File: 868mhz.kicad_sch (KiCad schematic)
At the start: 4 parts, among them J2 Conn_Coaxial, U2 RFM95W-868S2

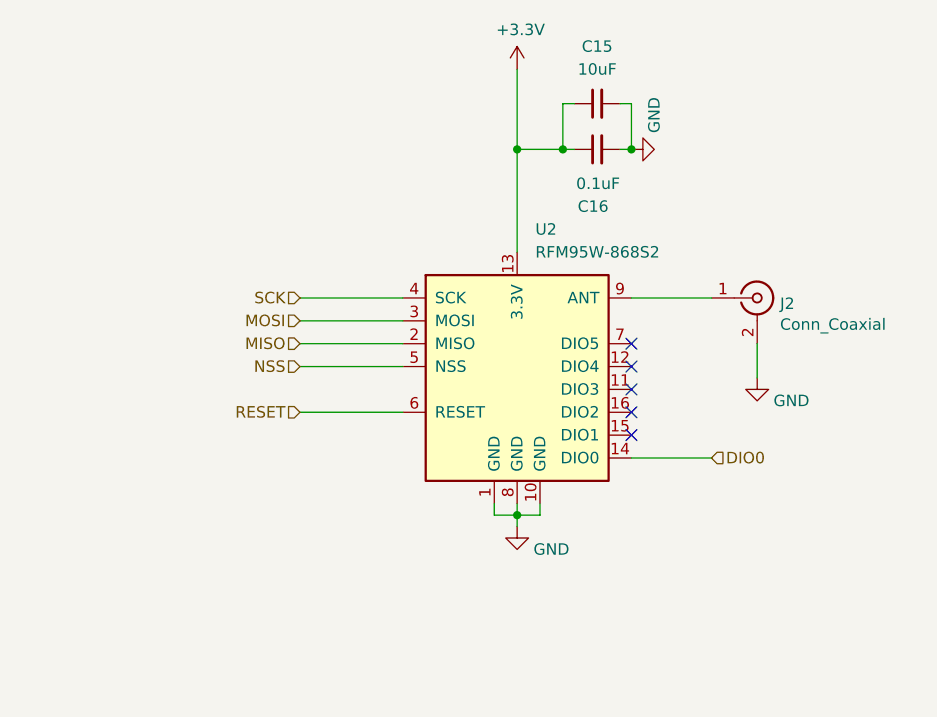
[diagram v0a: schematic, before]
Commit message: New Template Update
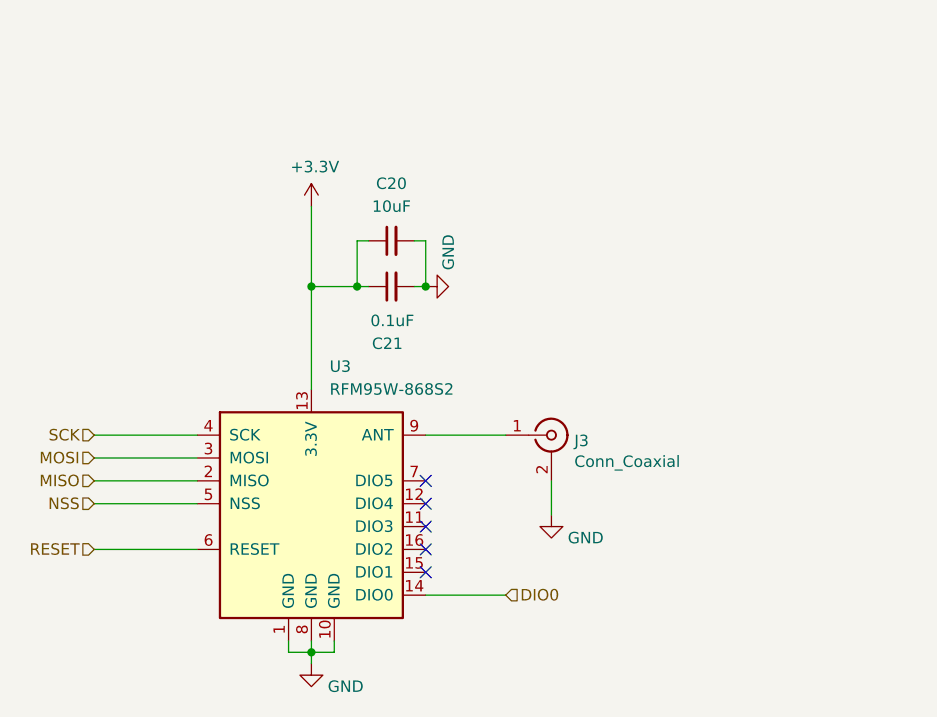
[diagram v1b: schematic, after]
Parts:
- removed C15: 10uF, Capacitor_SMD:C_0603_1608Metric, symbol Device:C_Small
- removed C16: 0.1uF, Capacitor_SMD:C_0603_1608Metric, symbol Device:C_Small
- removed J2: Conn_Coaxial, Connector_Coaxial:SMA_Molex_73251-1153_EdgeMount_Horizontal, symbol Connector:Conn_Coaxial
- removed U2: RFM95W-868S2, RF_Module:HOPERF_RFM9XW_SMD, symbol RF_Module:RFM95W-868S2
- added C20: 10uF, Capacitor_SMD:C_0402_1005Metric, symbol Device:C_Small
- added C21: 0.1uF, Capacitor_SMD:C_0402_1005Metric, symbol Device:C_Small
- added J3: Conn_Coaxial, Connector_Coaxial:SMA_Molex_73251-1153_EdgeMount_Horizontal, symbol Connector:Conn_Coaxial
- added U3: RFM95W-868S2, RF_Module:HOPERF_RFM9XW_SMD, symbol RF_Module:RFM95W-868S2
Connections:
- net +3V3: now also C20.1, C21.1, U3.13 (3.3V)
- net DIO0: now also U3.14 (DIO0)
- net GND: now also C20.2, C21.2, J3.2 (Ext), U3.1 (GND), U3.10 (GND), U3.8 (GND)
- net MISO: now also U3.2 (MISO)
- net MOSI: now also U3.3 (MOSI)
- net NSS: now also U3.5 (NSS)
- net RESET: now also U3.6 (RESET)
- net SCK: now also U3.4 (SCK)
- new net: J3.1 (In), U3.9 (ANT)
